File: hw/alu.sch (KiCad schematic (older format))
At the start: 3 parts

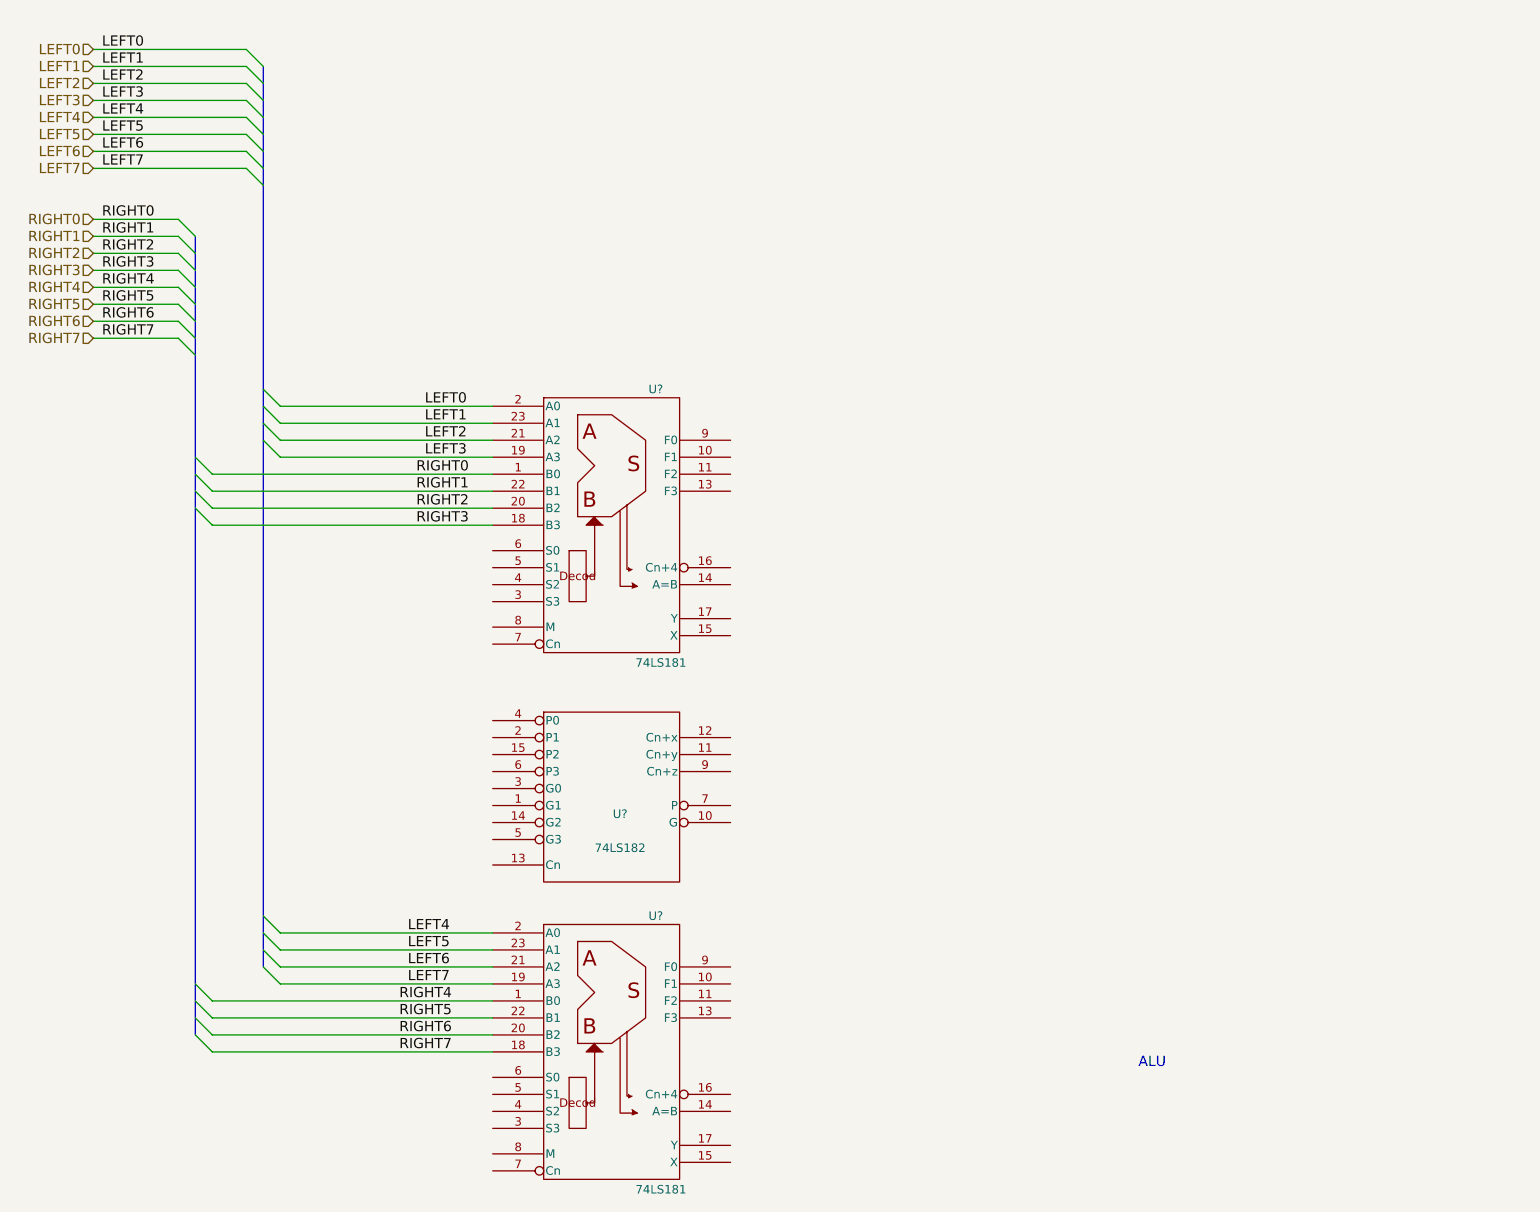
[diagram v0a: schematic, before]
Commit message: initial stab at ALU circuit
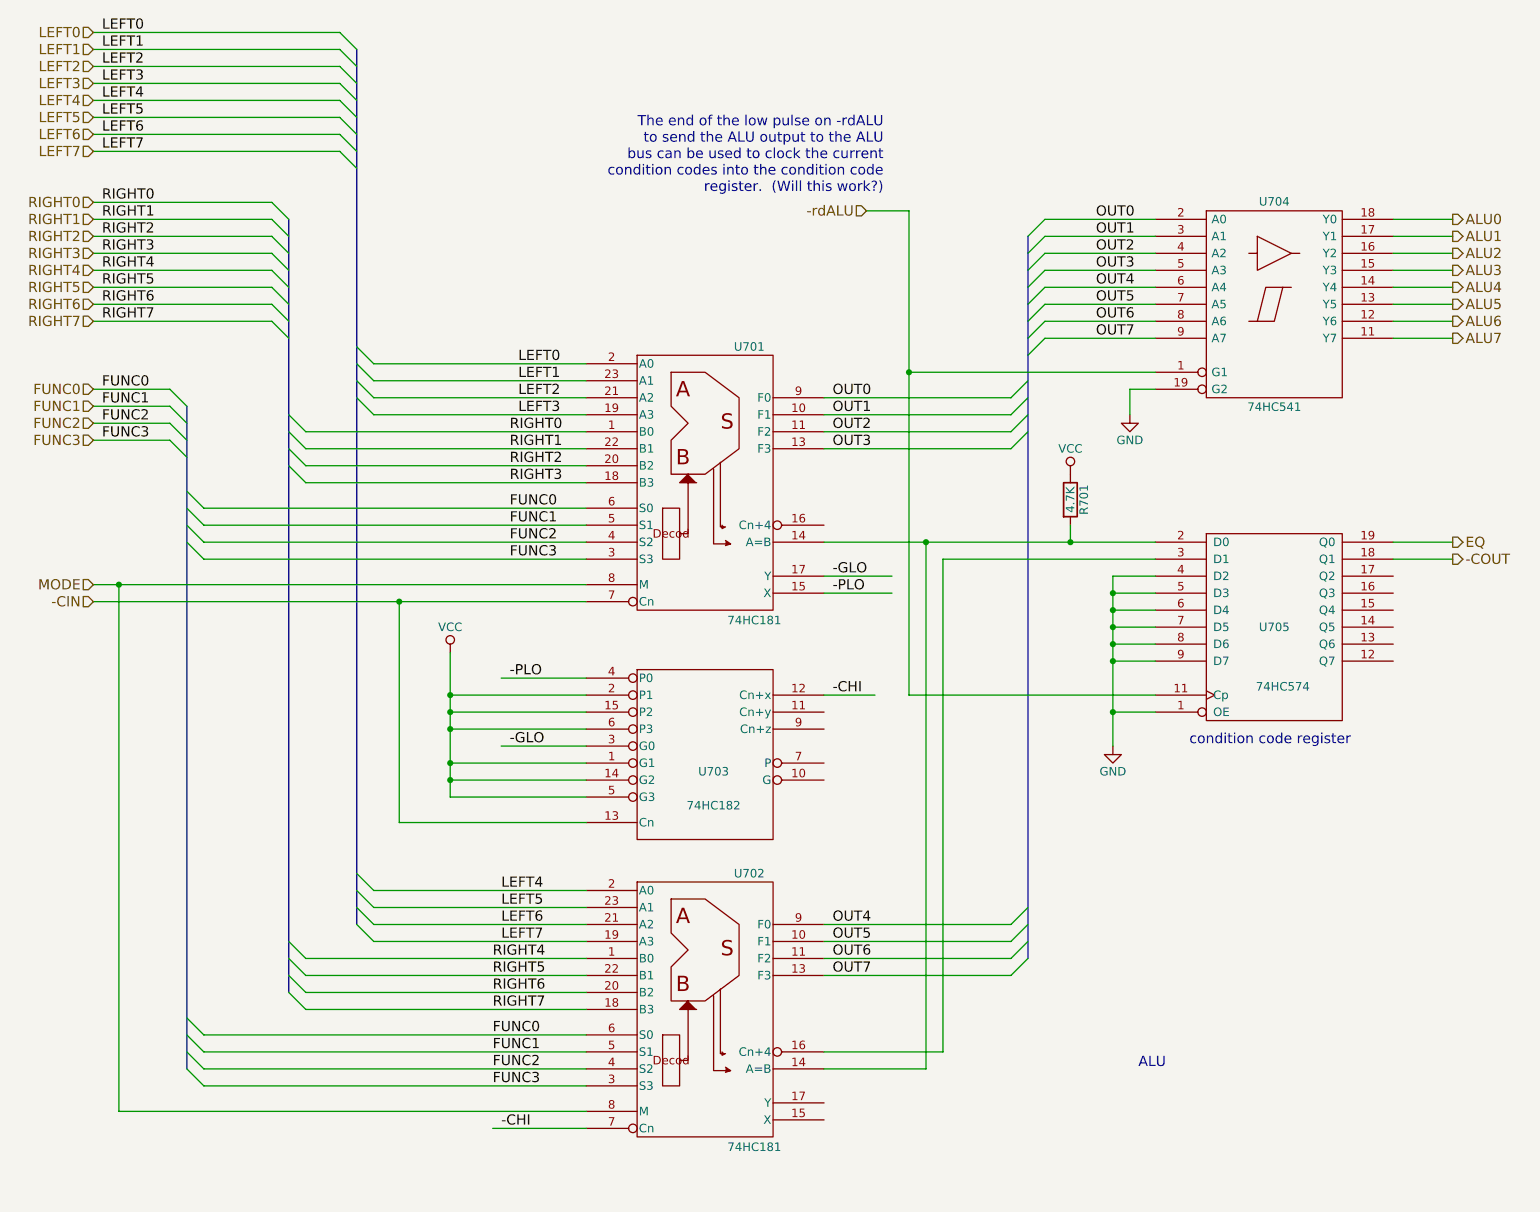
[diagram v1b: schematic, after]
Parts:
- added R701: 4.7K, symbol R
- added U704: 74HC541, symbol 74LS541
- added U705: 74HC574, symbol 74LS574
- U701, U702: renamed from U?; value 74LS181 -> 74HC181
- U703: renamed from U?; value 74LS182 -> 74HC182
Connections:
- net labels added: -CHI, -CIN, -COUT, -GLO, -PLO, -rdALU, ALU0, ALU1, ALU2, ALU3, ALU4, ALU5, ALU6, ALU7, EQ, FUNC0, FUNC1, FUNC2, FUNC3, GND, MODE, OUT0, OUT1, OUT2, OUT3, OUT4, OUT5, OUT6, OUT7, VCC
- wire segments 32 -> 110
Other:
- note added: "The end of the low pulse on -rdALU\nto send the ALU output to the ALU\nbus can be used to clock the current\ncondition codes into the condition code\nregister. (Will this work?)"
- note added: "condition code register"
- moved on the sheet: U701, U702, U703
